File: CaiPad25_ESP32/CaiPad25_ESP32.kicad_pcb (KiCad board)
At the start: 2 copper layers, 140 x 103 mm, 27 parts, among them J1 OLED_128x64, U1 ESP32_DevKit_V1_DOIT

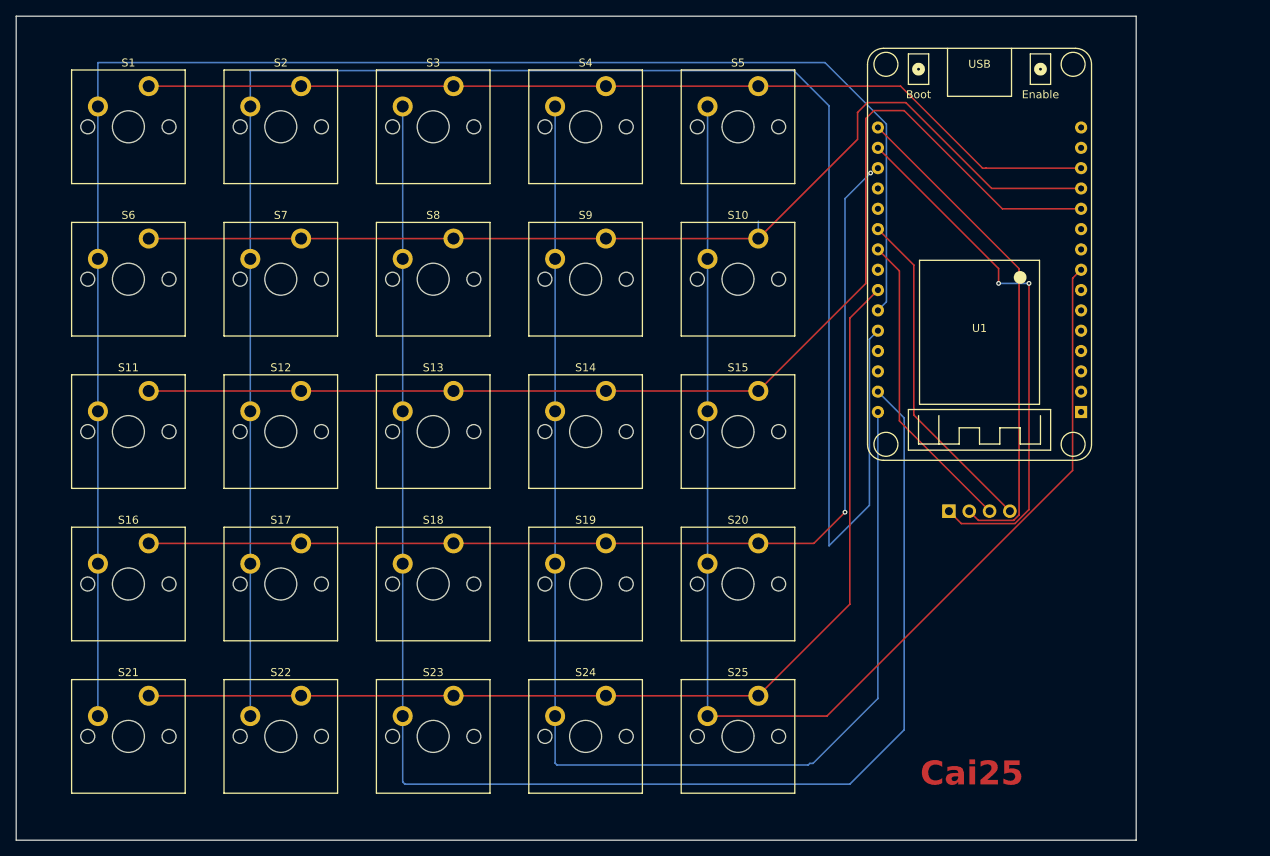
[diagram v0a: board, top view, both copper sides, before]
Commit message: update on CaiPad25_ESP32
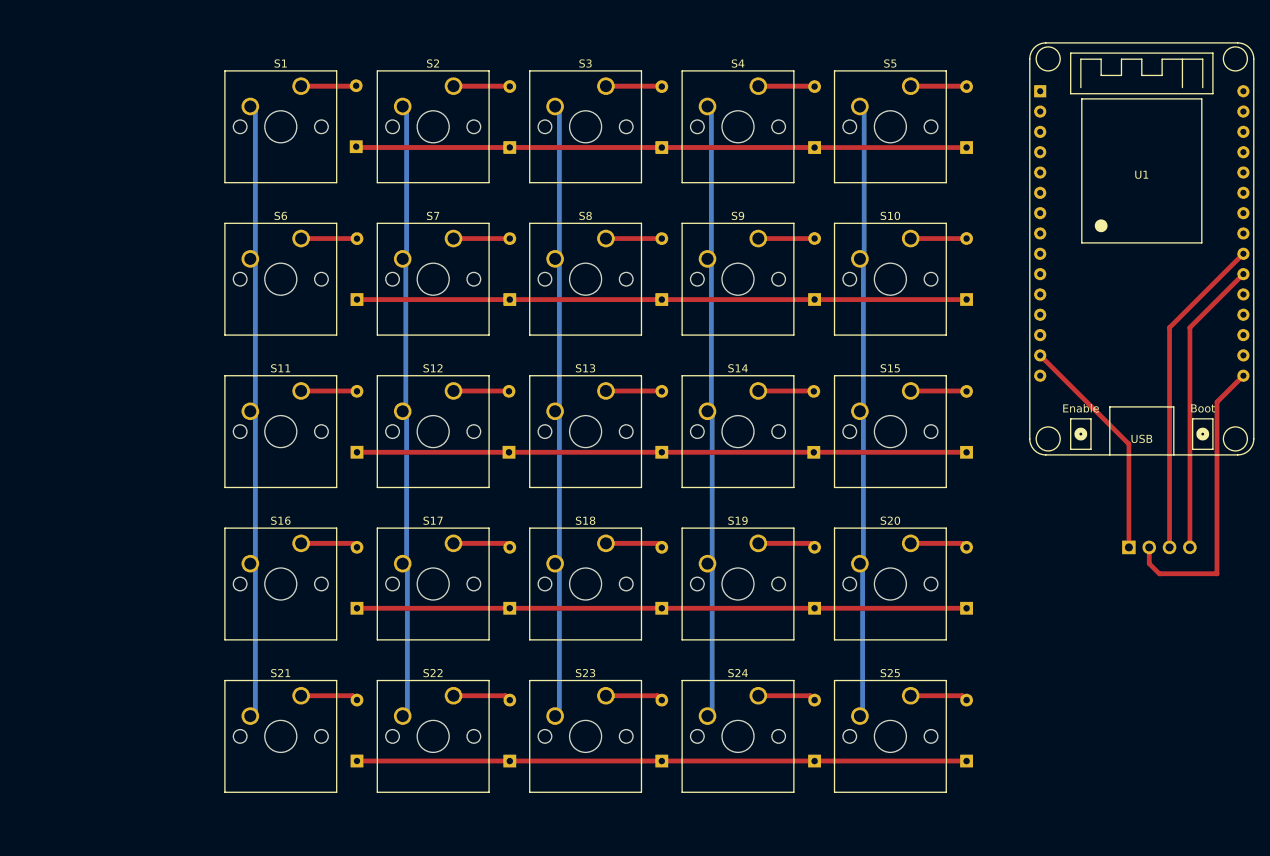
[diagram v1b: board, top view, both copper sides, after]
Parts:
- added D1: Diode, ScottoKeebs_Components:Diode_DO-35, B.Cu at (76.1, 50.1)
- added D10: Diode, ScottoKeebs_Components:Diode_DO-35, B.Cu at (152.4, 69.2)
- added D11: Diode, ScottoKeebs_Components:Diode_DO-35, B.Cu at (76.2, 88.3)
- added D12: Diode, ScottoKeebs_Components:Diode_DO-35, B.Cu at (95.2, 88.3)
- added D13: Diode, ScottoKeebs_Components:Diode_DO-35, B.Cu at (114.3, 88.3)
- added D14: Diode, ScottoKeebs_Components:Diode_DO-35, B.Cu at (133.3, 88.3)
- added D15: Diode, ScottoKeebs_Components:Diode_DO-35, B.Cu at (152.4, 88.3)
- added D16: Diode, ScottoKeebs_Components:Diode_DO-35, B.Cu at (76.2, 107.8)
- added D17: Diode, ScottoKeebs_Components:Diode_DO-35, B.Cu at (95.3, 107.8)
- added D18: Diode, ScottoKeebs_Components:Diode_DO-35, B.Cu at (114.3, 107.8)
- added D19: Diode, ScottoKeebs_Components:Diode_DO-35, B.Cu at (133.4, 107.8)
- added D2: Diode, ScottoKeebs_Components:Diode_DO-35, B.Cu at (95.3, 50.2)
- added D20: Diode, ScottoKeebs_Components:Diode_DO-35, B.Cu at (152.4, 107.8)
- added D21: Diode, ScottoKeebs_Components:Diode_DO-35, B.Cu at (76.2, 126.9)
- added D22: Diode, ScottoKeebs_Components:Diode_DO-35, B.Cu at (95.3, 126.9)
- added D23: Diode, ScottoKeebs_Components:Diode_DO-35, B.Cu at (114.3, 126.9)
- added D24: Diode, ScottoKeebs_Components:Diode_DO-35, B.Cu at (133.4, 126.9)
- added D25: Diode, ScottoKeebs_Components:Diode_DO-35, B.Cu at (152.4, 126.9)
- added D3: Diode, ScottoKeebs_Components:Diode_DO-35, B.Cu at (114.3, 50.2)
- added D4: Diode, ScottoKeebs_Components:Diode_DO-35, B.Cu at (133.4, 50.2)
- added D5: Diode, ScottoKeebs_Components:Diode_DO-35, B.Cu at (152.4, 50.2)
- added D6: Diode, ScottoKeebs_Components:Diode_DO-35, B.Cu at (76.2, 69.2)
- added D7: Diode, ScottoKeebs_Components:Diode_DO-35, B.Cu at (95.3, 69.2)
- added D8: Diode, ScottoKeebs_Components:Diode_DO-35, B.Cu at (114.3, 69.2)
- added D9: Diode, ScottoKeebs_Components:Diode_DO-35, B.Cu at (133.4, 69.2)
- S1, S10, S11, S12, S13, S14, S15, S16, S17, S18, S19, S2, S20, S21, S22, S23, S24, S25, S3, S4, S5, S6, S7, S8, S9: footprint ScottoKeebs_MX:MX_PCB_1.00u -> Button_Switch_Keyboard:SW_Cherry_MX_1.00u_PCB
- moved U1 44.9 mm to (174.3, 43.2), turned to 0 degrees
- moved J1 23.0 mm to (176.5, 100.2)
- moved S16 22.2 mm to (69.2, 99.7)
- moved S17 22.2 mm to (88.3, 99.7)
- moved S18 22.2 mm to (107.3, 99.7)
- moved S1 22.2 mm to (69.2, 42.5)
- moved S11 22.2 mm to (69.2, 80.6)
- moved S12 22.2 mm to (88.3, 80.6)
- moved S13 22.2 mm to (107.3, 80.6)
- moved S2 22.2 mm to (88.3, 42.5)
- moved S21 22.2 mm to (69.2, 118.7)
- moved S22 22.2 mm to (88.3, 118.7)
- moved S23 22.2 mm to (107.3, 118.7)
- moved S3 22.2 mm to (107.3, 42.5)
- moved S6 22.2 mm to (69.2, 61.6)
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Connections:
- S1 pad 1: Column 0 -> Net-(D1-A)
- S1 pad 2: Row 0 -> Column 0
- S10 pad 1: Column 4 -> Net-(D10-A)
- S10 pad 2: Row 1 -> Column 4
- S11 pad 1: Column 0 -> Net-(D11-A)
- S11 pad 2: Row 2 -> Column 0
- S12 pad 1: Column 1 -> Net-(D12-A)
- S12 pad 2: Row 2 -> Column 1
- S13 pad 1: Column 2 -> Net-(D13-A)
- S13 pad 2: Row 2 -> Column 2
- S14 pad 1: Column 3 -> Net-(D14-A)
- S14 pad 2: Row 2 -> Column 3
- S15 pad 1: Column 4 -> Net-(D15-A)
- S15 pad 2: Row 2 -> Column 4
- S16 pad 1: Column 0 -> Net-(D16-A)
- S16 pad 2: Row 3 -> Column 0
- S17 pad 1: Column 1 -> Net-(D17-A)
- S17 pad 2: Row 3 -> Column 1
- S18 pad 1: Column 2 -> Net-(D18-A)
- S18 pad 2: Row 3 -> Column 2
- S19 pad 1: Column 3 -> Net-(D19-A)
- S19 pad 2: Row 3 -> Column 3
- S2 pad 1: Column 1 -> Net-(D2-A)
- S2 pad 2: Row 0 -> Column 1
- S20 pad 1: Column 4 -> Net-(D20-A)
- S20 pad 2: Row 3 -> Column 4
- S21 pad 1: Column 0 -> Net-(D21-A)
- S21 pad 2: Row 4 -> Column 0
- S22 pad 1: Column 1 -> Net-(D22-A)
- S22 pad 2: Row 4 -> Column 1
- S23 pad 1: Column 2 -> Net-(D23-A)
- S23 pad 2: Row 4 -> Column 2
- S24 pad 1: Column 3 -> Net-(D24-A)
- S24 pad 2: Row 4 -> Column 3
- S25 pad 1: Column 4 -> Net-(D25-A)
- S25 pad 2: Row 4 -> Column 4
- S3 pad 1: Column 2 -> Net-(D3-A)
- S3 pad 2: Row 0 -> Column 2
- S4 pad 1: Column 3 -> Net-(D4-A)
- S4 pad 2: Row 0 -> Column 3
- S5 pad 1: Column 4 -> Net-(D5-A)
- S5 pad 2: Row 0 -> Column 4
- S6 pad 1: Column 0 -> Net-(D6-A)
- S6 pad 2: Row 1 -> Column 0
- S7 pad 1: Column 1 -> Net-(D7-A)
- S7 pad 2: Row 1 -> Column 1
- S8 pad 1: Column 2 -> Net-(D8-A)
- S8 pad 2: Row 1 -> Column 2
- S9 pad 1: Column 3 -> Net-(D9-A)
- S9 pad 2: Row 1 -> Column 3
- U1 pad 10: unconnected-(U1-IO27-Pad10) -> Column 1
- U1 pad 11: Row 2 -> Column 2
- U1 pad 12: Row 1 -> Column 3
- U1 pad 13: Row 0 -> Column 4
- U1 pad 14: unconnected-(U1-GND-Pad14) -> Net-(J1-GND)
- U1 pad 17: Net-(J1-GND) -> unconnected-(U1-GND-Pad17)
- U1 pad 18: Row 3 -> Row 0
- U1 pad 19: unconnected-(U1-IO2-Pad19) -> Row 1
- U1 pad 24: Row 4 -> Row 2
- U1 pad 25: Column 0 -> Row 3
- U1 pad 26: Column 1 -> Row 4
- U1 pad 29: Column 2 -> unconnected-(U1-IO22-Pad29)
- U1 pad 30: Column 3 -> unconnected-(U1-IO23-Pad30)
- U1 pad 8: Column 4 -> unconnected-(U1-IO25-Pad8)
- U1 pad 9: unconnected-(U1-IO26-Pad9) -> Column 0
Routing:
- net Column 1: track 239.4 -> 77.8 mm
- net Column 0: track 207.2 -> 78.3 mm
- net Column 2: track 193.7 -> 78.0 mm
- net Column 3: track 161.8 -> 78.0 mm
- net Column 4: track 160.1 -> 77.6 mm
- net Row 2: track 148.2 -> 76.2 mm
- net Row 4: track 133.1 -> 76.2 mm
- net Row 3: track 132.4 -> 76.2 mm, vias 2 -> 0
- net Row 1: track 132.2 -> 76.2 mm
- net Row 0: track 120.8 -> 76.3 mm
- net Net-(J1-GND): track 66.6 -> 28.6 mm, vias 2 -> 0
- net Net-(J1-VCC): track 62.7 -> 37.2 mm
- net Net-(D24-A): track 0.00 -> 7.26 mm
- net Net-(D22-A): track 0.00 -> 7.26 mm
- net Net-(D19-A): track 0.00 -> 7.24 mm
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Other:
- board outline removed
- board text removed: "Cai25"
